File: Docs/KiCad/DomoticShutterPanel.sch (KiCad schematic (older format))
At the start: 35 parts, among them J1 Conn_01x12, J10 Conn_01x03, J11 Conn_01x03, J12 Conn_01x03, J13 Conn_01x03, J14 Conn_01x03, J15 Conn_01x04, J2 Conn_01x12, J3 Conn_01x06, J4 Conn_01x02, J5 Conn_01x02, J6 Conn_01x02, J7 3.3V DC-DC Step-Down Power Mo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, J8 Conn_01x03, J9 Conn_01x03, K1 SRD-05VDC-SL-C, K2 SRD-05VDC-SL-C, K3 SRD-05VDC-SL-C, K4 SRD-05VDC-SL-C, K5 SRD-05VDC-SL-C, K6 SRD-05VDC-SL-C, K7 SRD-05VDC-SL-C, SW1 SW_Push, SW2 SW_Push, SW3 SW_Push, SW4 SW_Push, U1 ULN2803A

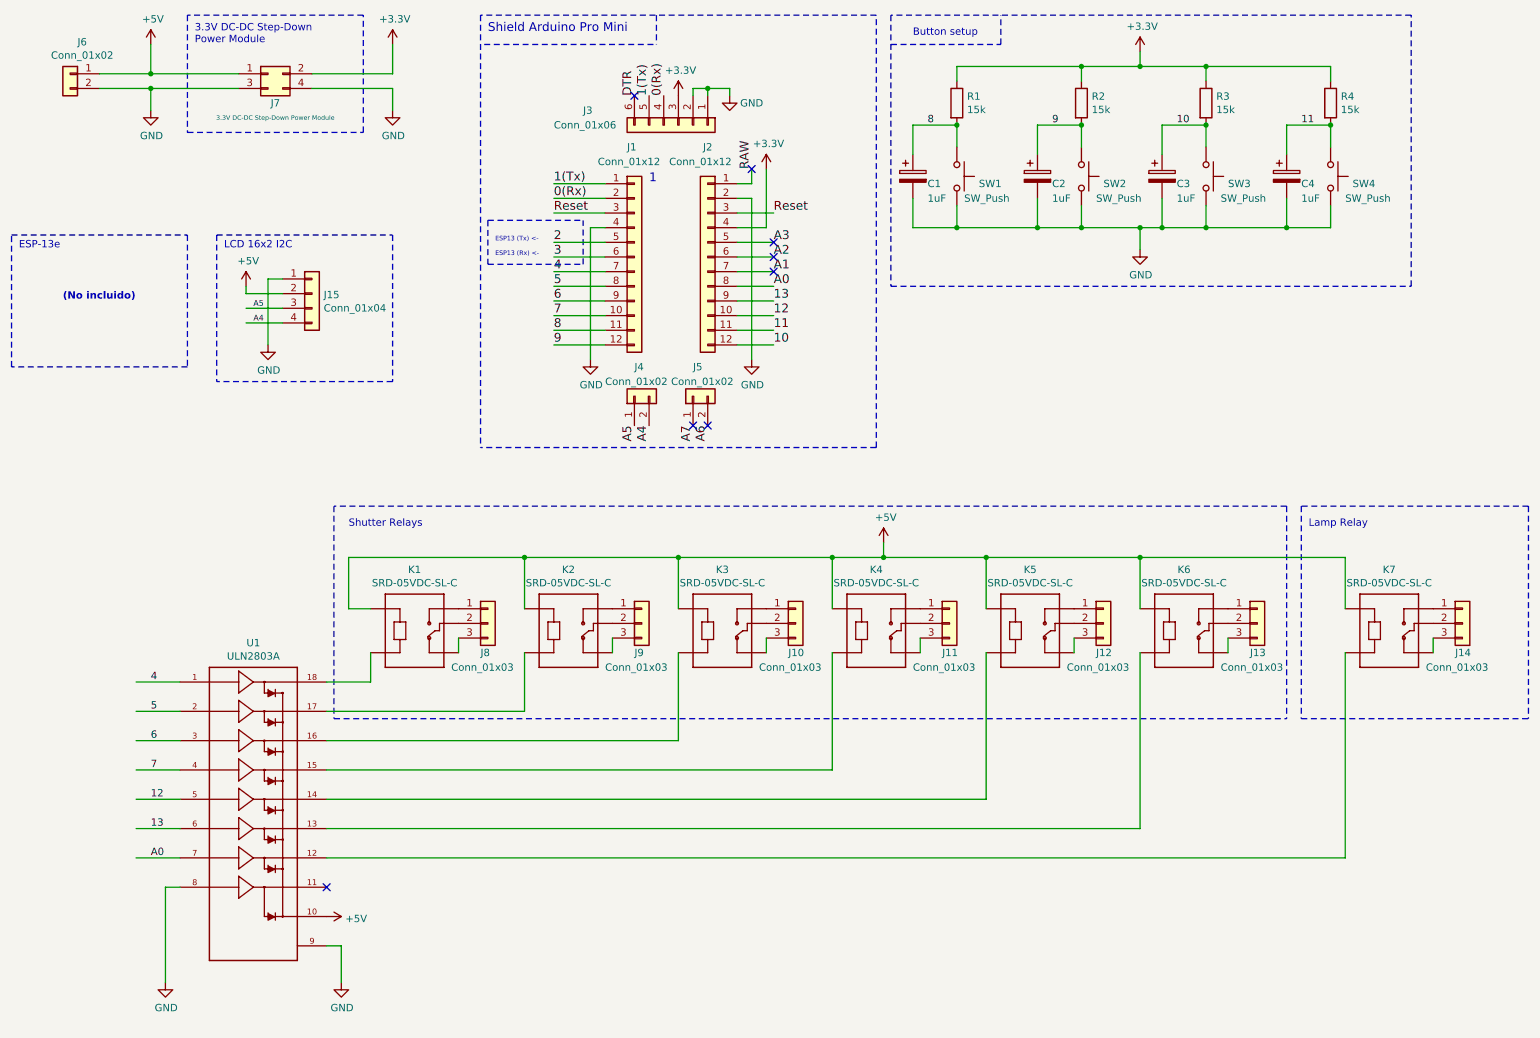
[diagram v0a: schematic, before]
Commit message: Changed to radio approach
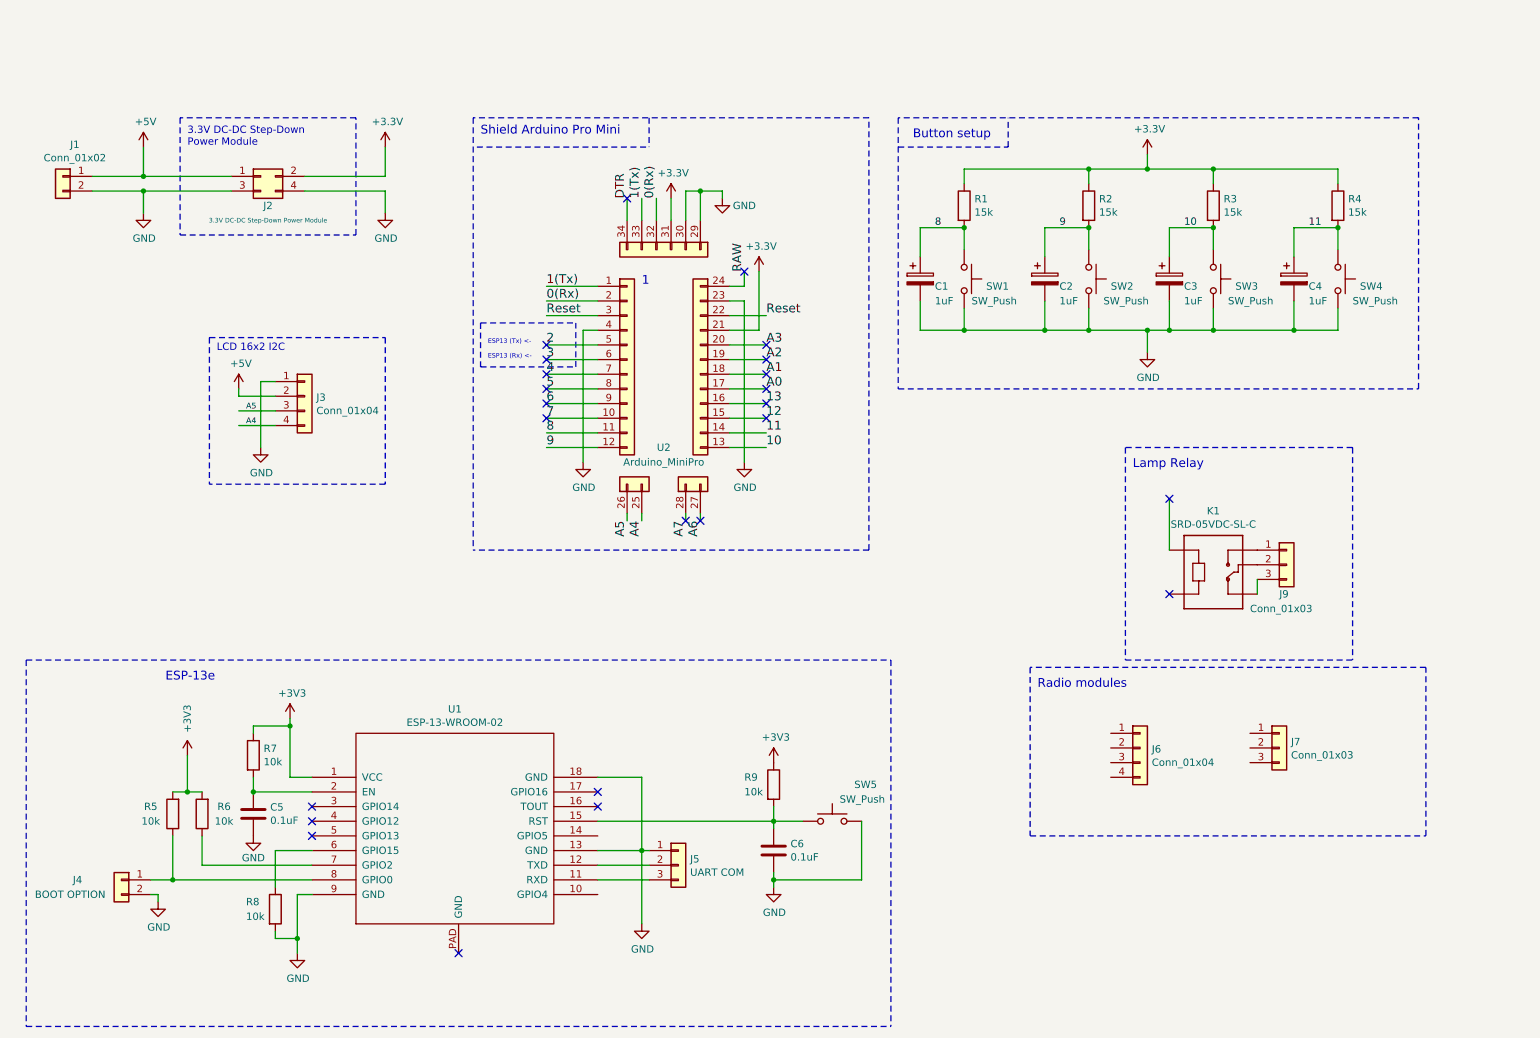
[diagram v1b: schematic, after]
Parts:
- removed J1, J2: Conn_01x12, Custom_libraries:Socket_Strip_Arduino_1x12, symbol CustomLibraries_connectors:Conn_01x12
- removed J10, J11, J12, J13, J8, J9: Conn_01x03, Custom_libraries:ScrewTerminal_01X03_5mm, symbol CustomLibraries_connectors:Conn_01x03
- removed J3: Conn_01x06, Custom_libraries:Socket_Strip_Arduino_1x06, symbol CustomLibraries_connectors:Conn_01x06
- removed J5: Conn_01x02, Custom_libraries:Socket_Strip_Arduino_1x02, symbol CustomLibraries_connectors:Conn_01x02
- removed K1, K2, K3, K4, K5, K6: SRD-05VDC-SL-C, symbol CustomLibraries_SRD-05VDC-SL-C:SRD-05VDC-SL-C
- removed U1: ULN2803A, symbol CustomLibraries_ULN2803A:ULN2803A
- added C5, C6: 0.1uF, symbol CustomLibraries_Device:C
- added J5: UART COM, symbol CustomLibraries_connectors:Conn_01x03
- added J6: Conn_01x04, symbol CustomLibraries_connectors:Conn_01x04
- added J7: Conn_01x03, symbol CustomLibraries_connectors:Conn_01x03
- added R5, R6, R7, R8, R9: 10k, symbol CustomLibraries_Device:R
- added SW5: SW_Push, symbol CustomLibraries_Switch:SW_Push
- added U1: ESP-13-WROOM-02, Custom_libraries:ESP-13-WROOM-02, symbol ESP8266:ESP-13-WROOM-02
- added U2: Arduino_MiniPro, Custom_libraries:Socket_Strip_Arduino_MiniPro, symbol CustomLibraries_connectors:Arduino_MiniPro
- J4: value Conn_01x02 -> BOOT OPTION; footprint Custom_libraries:Socket_Strip_Arduino_1x02 -> (none)
- renumbered J6 to J1, J7 to J2, J15 to J3, J14 to J9, K7 to K1
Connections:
- net labels added: +3V3
- wire segments 135 -> 136
- no-connect marks 8 -> 24
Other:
- note added: "Radio modules"
- note removed: "(No incluido)"
- note removed: "Shutter Relays"
- moved on the sheet: C1, C2, C3, C4, J1, J2, J3, J9, K1, R1, R2, R3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
